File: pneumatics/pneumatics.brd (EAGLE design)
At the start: 46.7 x 38.1 mm, 26 parts, among them U1 TPIC6A596

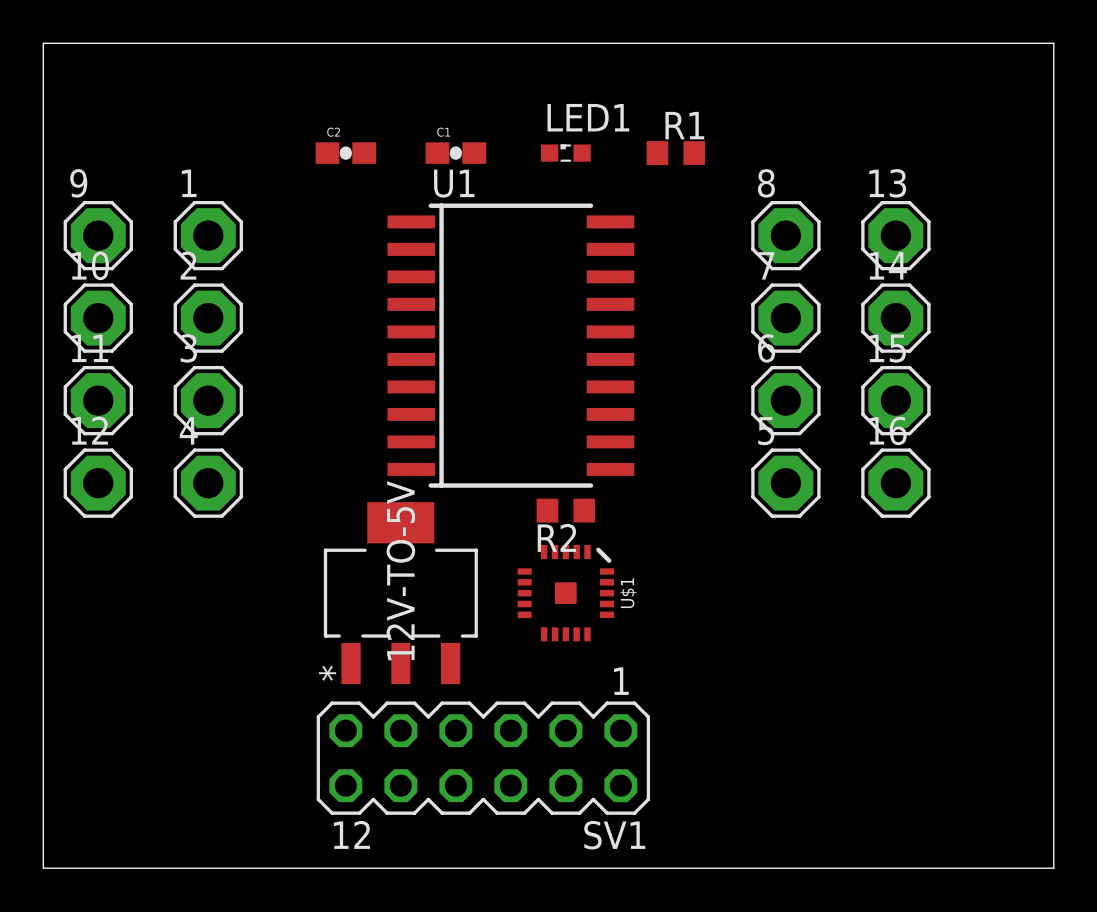
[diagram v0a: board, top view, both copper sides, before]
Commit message: Intermediate board
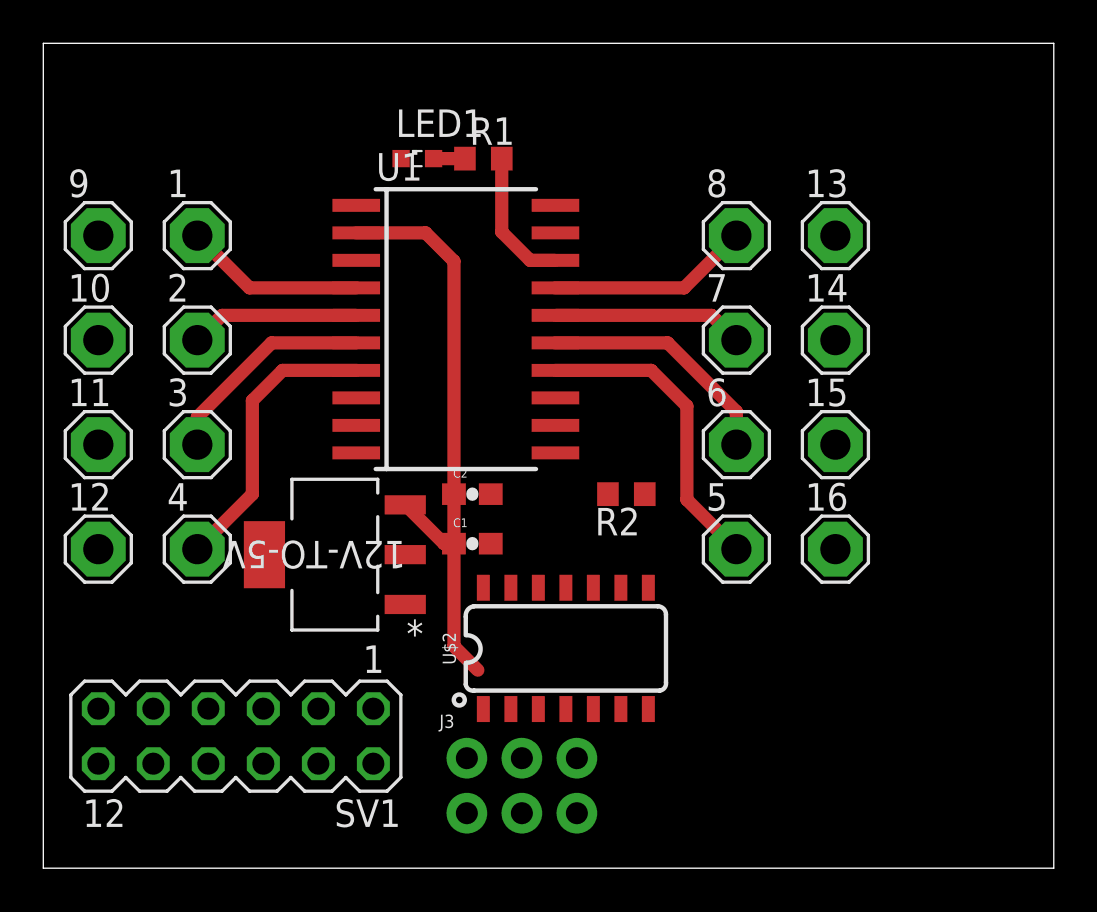
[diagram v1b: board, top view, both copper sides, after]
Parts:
- removed U$1: ATTINY84ATTINY84-20MU, SparkFun-IC-Microcontroller:QFN20
- added J3: AVR_SPI_PROG_3X2NS, SparkFun-Connectors:2X3-NS
- added U$2: ATTINY84, SparkFun-IC-Microcontroller:SO14
- moved C1 18.1 mm to (19.8, 15.0)
- moved C2 16.8 mm to (19.8, 17.3)
- moved SV1 11.5 mm to (8.89, 6.10)
- moved R1 8.89 mm to (20.3, 32.8)
- moved LED1 6.86 mm to (17.3, 32.8)
- moved 16 4.13 mm to (36.6, 14.7)
- moved 5 3.81 mm to (32.0, 14.7)
- moved 12V-TO-5V 3.53 mm to (13.5, 14.5), turned to 180 degrees
- moved 15 3.45 mm to (36.6, 19.6)
- moved 4 3.09 mm to (7.11, 14.7)
- moved 6 3.06 mm to (32.0, 19.6)
- moved 12 3.05 mm to (2.54, 14.7)
- moved 14 2.97 mm to (36.6, 24.4)
- moved R2 2.90 mm to (26.9, 17.3)
- moved 13 2.79 mm to (36.6, 29.2)
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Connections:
- removed net ENABLE: U$1.20, U1.9
- removed net SCL: SV1.2, U$1.1
- removed net SDA: SV1.1, U$1.16
- new net ENABLE/MISO: J3.1, U$2.8, U1.9
- new net RESET: J3.5, U$2.4
- new net SCL/SCK: J3.3, SV1.2, U$2.9
- new net SDA/MOSI: J3.4, SV1.1, U$2.7
- net +5V: now also J3.2, U$2.1; no longer U$1.9
- net GND: now also J3.6, U$2.14; no longer U$1.8
- net RCLK: now also U$2.12; no longer U$1.2
- net SERIAL_IN: now also U$2.13; no longer U$1.5
- net SRCLK: now also U$2.10; no longer U$1.4
- net SRCLR: now also U$2.11; no longer U$1.3
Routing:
- net +5V: track 0.00 -> 27.4 mm
- net SOL_3A: track 0.00 -> 14.3 mm
- net SOL_2B: track 0.00 -> 13.3 mm
- net SOL_3B: track 0.00 -> 11.2 mm
- net SOL_2A: track 0.00 -> 10.0 mm
- net SOL_4B: track 0.00 -> 9.35 mm
- net SOL_4A: track 0.00 -> 8.83 mm
- net SOL_1A: track 0.00 -> 8.34 mm
- net SOL_1B: track 0.00 -> 7.81 mm
- net N$1: track 0.00 -> 6.41 mm
- net N$7: track 0.00 -> 1.45 mm
